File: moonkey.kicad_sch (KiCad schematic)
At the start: 36 parts, among them J1 AudioJack4, SW1 SW_Push, SW10 SW_Push, SW11 SW_Push, SW12 SW_Push, SW13 SW_Push, SW14 SW_Push, SW15 SW_Push, SW16 SW_Push, SW17 SW_Push, SW2 SW_Push, SW3 SW_Push, SW4 SW_Push, SW5 SW_Push, SW6 SW_Push, SW7 SW_Push, SW8 SW_Push, SW9 SW_Push

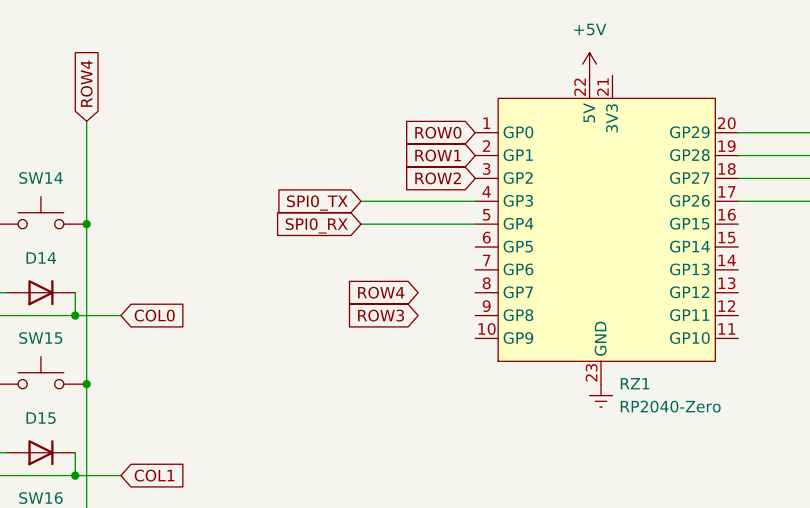
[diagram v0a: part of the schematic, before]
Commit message: uptate: ortholinear
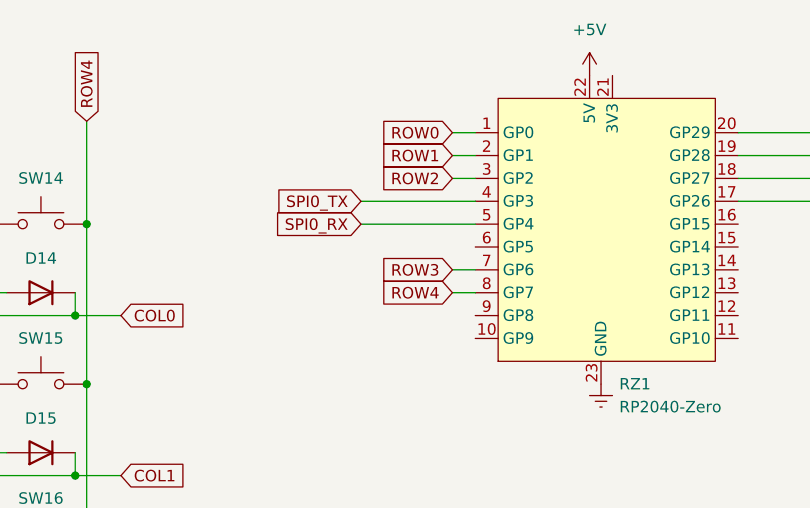
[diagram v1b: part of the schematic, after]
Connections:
- net ROW3: now also RZ1.7 (GP6)
- net ROW4: now also RZ1.8 (GP7)
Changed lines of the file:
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@@
+    (stroke (width 0) (type default) (color 0 0 0 0))
+  )
+  (wire (pts (xy 151.13 86.36) (xy 153.67 86.36))
     (stroke (width 0) (type default) (color 0 0 0 0))
   )
@@
     (stroke (width 0) (type default) (color 0 0 0 0))
   )
+  (wire (pts (xy 151.13 71.12) (xy 153.67 71.12))
+    (stroke (width 0) (type default) (color 0 0 0 0))
+  )
   (wire (pts (xy 54.61 106.68) (xy 55.88 106.68))
     (stroke (width 0) (type default) (color 0 0 0 0))
@@
     (stroke (width 0) (type default) (color 0 0 0 0))
   )
+  (wire (pts (xy 151.13 73.66) (xy 153.67 73.66))
+    (stroke (width 0) (type default) (color 0 0 0 0))
+  )
   (wire (pts (xy 54.61 81.28) (xy 54.61 88.9))
     (stroke (width 0) (type default) (color 0 0 0 0))
@@
     (stroke (width 0) (type default) (color 0 0 0 0))
   )
+  (wire (pts (xy 151.13 88.9) (xy 153.67 88.9))
+    (stroke (width 0) (type default) (color 0 0 0 0))
+  )
   (wire (pts (xy 48.26 124.46) (xy 48.26 127))
     (stroke (width 0) (type default) (color 0 0 0 0))
@@
     (stroke (width 0) (type default) (color 0 0 0 0))
   )
+  (wire (pts (xy 151.13 76.2) (xy 153.67 76.2))
+    (stroke (width 0) (type default) (color 0 0 0 0))
+  )
   (wire (pts (xy 109.22 127) (xy 114.3 127))
     (stroke (width 0) (type default) (color 0 0 0 0))
@@
     )
   )
-  (global_label "ROW0" (shape input) (at 153.67 71.12 180) (fields_autoplaced)
-    (effects (font (size 1.27 1.27)) (justify right))
-    (property "시트 간 참조" "${INTERSHEET_REFS}" (id 0) (at 145.9955 71.0406 0)
+  (global_label "ROW0" (shape input) (at 151.13 71.12 180) (fields_autoplaced)
+    (effects (font (size 1.27 1.27)) (justify right))
+    (property "시트 간 참조" "${INTERSHEET_REFS}" (id 0) (at 143.4555 71.0406 0)
       (effects (font (size 1.27 1.27)) (justify right) hide)
     )
@@
     )
   )
-  (global_label "ROW1" (shape input) (at 153.67 73.66 180) (fields_autoplaced)
-    (effects (font (size 1.27 1.27)) (justify right))
-    (property "시트 간 참조" "${INTERSHEET_REFS}" (id 0) (at 145.9955 73.5806 0)
+  (global_label "ROW1" (shape input) (at 151.13 73.66 180) (fields_autoplaced)
+    (effects (font (size 1.27 1.27)) (justify right))
+    (property "시트 간 참조" "${INTERSHEET_REFS}" (id 0) (at 143.4555 73.5806 0)
       (effects (font (size 1.27 1.27)) (justify right) hide)
     )
@@
     )
   )
-  (global_label "ROW3" (shape input) (at 147.32 91.44 180) (fields_autoplaced)
-    (effects (font (size 1.27 1.27)) (justify right))
-    (property "시트 간 참조" "${INTERSHEET_REFS}" (id 0) (at 139.6455 91.3606 0)
+  (global_label "ROW3" (shape input) (at 151.13 86.36 180) (fields_autoplaced)
+    (effects (font (size 1.27 1.27)) (justify right))
+    (property "시트 간 참조" "${INTERSHEET_REFS}" (id 0) (at 143.4555 86.2806 0)
       (effects (font (size 1.27 1.27)) (justify right) hide)
     )
@@
     )
   )
-  (global_label "ROW2" (shape input) (at 153.67 76.2 180) (fields_autoplaced)
-    (effects (font (size 1.27 1.27)) (justify right))
-    (property "시트 간 참조" "${INTERSHEET_REFS}" (id 0) (at 145.9955 76.1206 0)
+  (global_label "ROW2" (shape input) (at 151.13 76.2 180) (fields_autoplaced)
+    (effects (font (size 1.27 1.27)) (justify right))
+    (property "시트 간 참조" "${INTERSHEET_REFS}" (id 0) (at 143.4555 76.1206 0)
       (effects (font (size 1.27 1.27)) (justify right) hide)
     )
@@
     )
   )
-  (global_label "ROW4" (shape input) (at 147.32 88.9 180) (fields_autoplaced)
-    (effects (font (size 1.27 1.27)) (justify right))
-    (property "시트 간 참조" "${INTERSHEET_REFS}" (id 0) (at 139.6455 88.8206 0)
-      (effects (font (size 1.27 1.27)) (justify right) hide)
-    )
+  (global_label "ROW4" (shape input) (at 151.13 88.9 180) (fields_autoplaced)
+    (effects (font (size 1.27 1.27)) (justify right))
+    (property "시트 간 참조" "${INTERSHEET_REFS}" (id 0) (at 143.4555 88.8206 0)
+      (effects (font (size 1.27 1.27)) (justify right) hide)
+    )
